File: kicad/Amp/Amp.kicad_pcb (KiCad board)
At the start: 2 copper layers, 30 x 25.6 mm, 23 parts, among them J1 Conn, J2 Conn, J3 Conn, J4 Conn, J5 Conn, J6 Conn, Q1 Q_NPN_BEC, U1 AD8541, U2 TS5A3166DBVR, U3 MCP1700

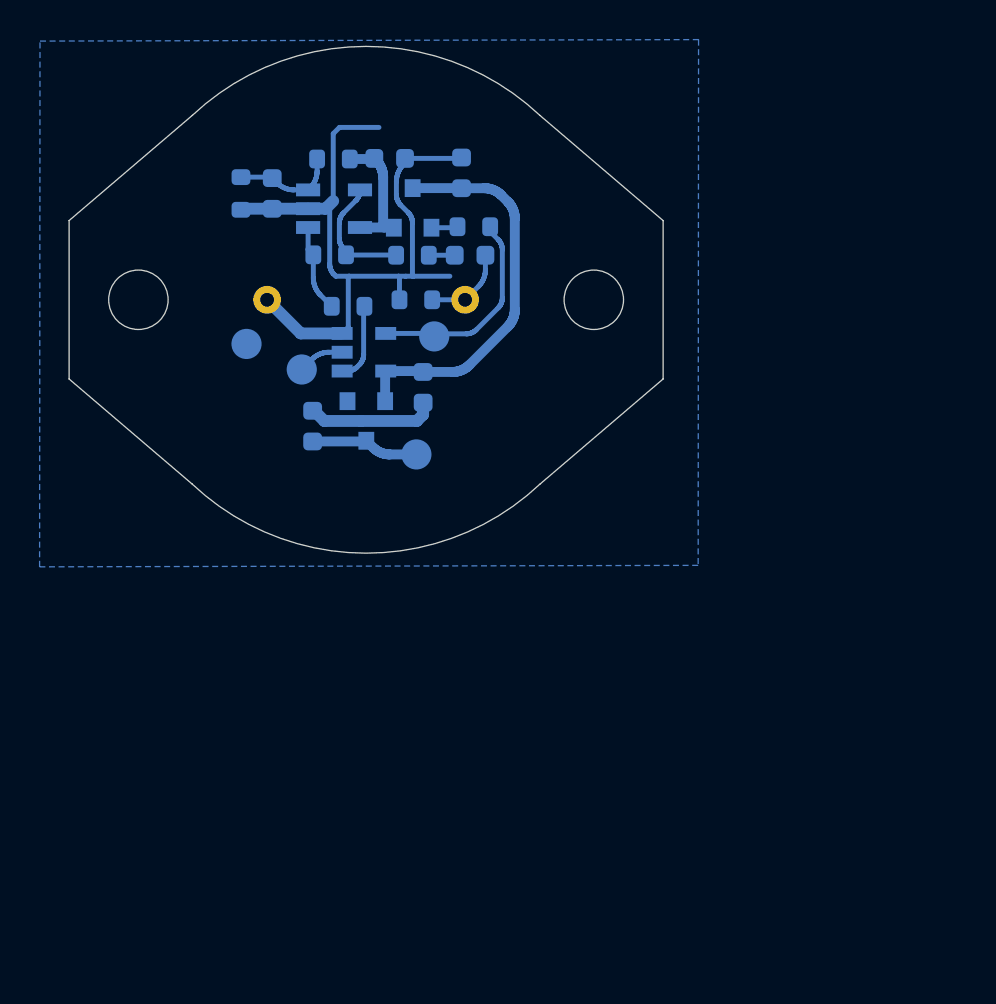
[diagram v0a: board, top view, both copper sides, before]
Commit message: изменено:      kicad/Amp/Amp-cache.lib 	изменено:      kicad/Amp/Amp.kicad_pcb 	изменено:      kicad/Amp/Amp.kicad_pcb-bak 	изменено:      kicad/Amp/Amp.sch 	изменено:      kicad/Amp/Amp.sch-bak 	изменено:      stm32cubeide/Anemometr_v3/Core/Src/main.c 	изменено:      stm32cubeide/Anemometr_v3/Core/Src/stm32f1xx_it.c 	изменено:      stm32cubeide/Anemometr_v3/Debug/Anemometr_3.bin 	изменено:      stm32cubeide/Anemometr_v3/Debug/Anemometr_3.elf 	изменено:      stm32cubeide/Anemometr_v3/Debug/Anemometr_3.list 	изменено:      stm32cubeide/Anemometr_v3/Debug/Anemometr_3.map 	изменено:      stm32cubeide/Anemometr_v3/Debug/Core/Src/main.o 	изменено:      stm32cubeide/Anemometr_v3/Debug/Core/Src/main.su 	изменено:      stm32cubeide/Anemometr_v3/Debug/Core/Src/stm32f1xx_it.o 	изменено:      stm32cubeide/Anemometr_v3/Release/Anemometr_3.bin 	изменено:      stm32cubeide/Anemometr_v3/Release/Anemometr_3.elf 	изменено:      stm32cubeide/Anemometr_v3/Release/Anemometr_3.list 	изменено:      stm32cubeide/Anemometr_v3/Release/Anemometr_3.map 	изменено:      stm32cubeide/Anemometr_v3/Release/Core/Src/main.o 	изменено:      stm32cubeide/Anemometr_v3/Release/Core/Src/main.su 	изменено:      stm32cubeide/Anemometr_v3/Release/Core/Src/stm32f1xx_it.o
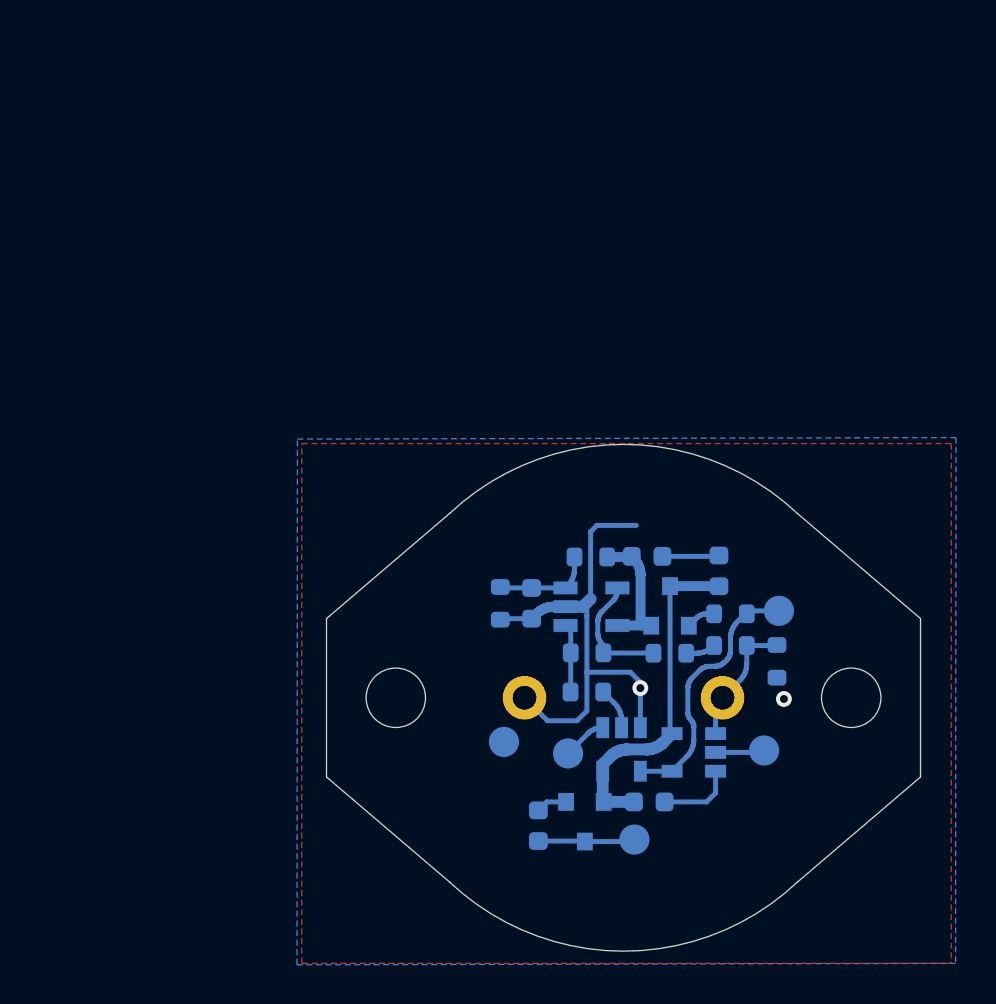
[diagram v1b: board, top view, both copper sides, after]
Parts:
- added J7: Conn, My-library:SMD-CONN, B.Cu at (50.1, 80.3)
- added U4: TS5A3167DBVR, Package_TO_SOT_SMD:SOT-23-5, B.Cu at (46.5, 80.5)
- C1: footprint Capacitor_SMD:C_0603_1608Metric -> Resistor_SMD:R_0603_1608Metric
- J1, J2: footprint Connector_Pin:Pin_D0.7mm_L6.5mm_W1.8mm_FlatFork -> My-library:connBig
- moved R6 25.8 mm to (50.8, 75.8), turned to 270 degrees
- moved C3 24.5 mm to (38.4, 72.9)
- moved R3 24.5 mm to (36.8, 72.9)
- moved C5 23.9 mm to (47.8, 71.3)
- moved J6 23.9 mm to (37.0, 79.9)
- moved R2 23.9 mm to (41.4, 70.6)
- moved R4 23.9 mm to (41.2, 75.4)
- moved U1 23.9 mm to (41.4, 73.1)
- moved C2 23.9 mm to (44.2, 70.5)
- moved J1 23.9 mm to (48.0, 77.7)
- moved J2 23.9 mm to (38.0, 77.7)
- moved Q1 23.9 mm to (45.4, 73.0)
- moved R1 23.9 mm to (45.3, 75.4)
- moved U2 23.9 mm to (42.9, 80.3), turned to 270 degrees
- moved C6 23.9 mm to (44.3, 83.0), turned to 0 degrees
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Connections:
- net Net-(C5-Pad1) renamed /3.3v
- U2 pad 1: Net-(C4-Pad1) -> /Out
- U2 pad 2: /Out -> Net-(C4-Pad1)
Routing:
- net GND: track 45.0 -> 34.9 mm, vias 0 -> 2
- net /Select: track 10.6 -> 13.3 mm
- net /3.3v: track 20.1 -> 17.4 mm
- net /Signal: track 0.00 -> 2.49 mm
- net /In: track 4.29 -> 6.59 mm
- net Net-(C4-Pad1): track 4.00 -> 2.13 mm
- net Net-(C4-Pad2): track 4.42 -> 3.47 mm
- net /+5v: track 5.49 -> 4.90 mm
- added copper zone on F.Cu, net GND
